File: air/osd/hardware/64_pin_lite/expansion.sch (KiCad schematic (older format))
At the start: 7 parts, among them P11 CONN_1, P13 CONN_1, P2 CONN_20, P3 CONN_20

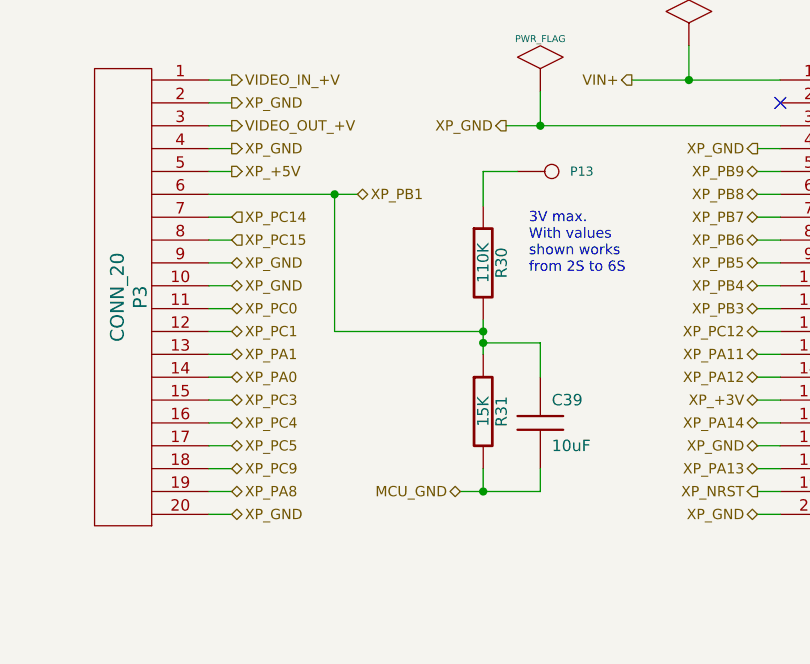
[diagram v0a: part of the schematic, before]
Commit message: hopefully finished
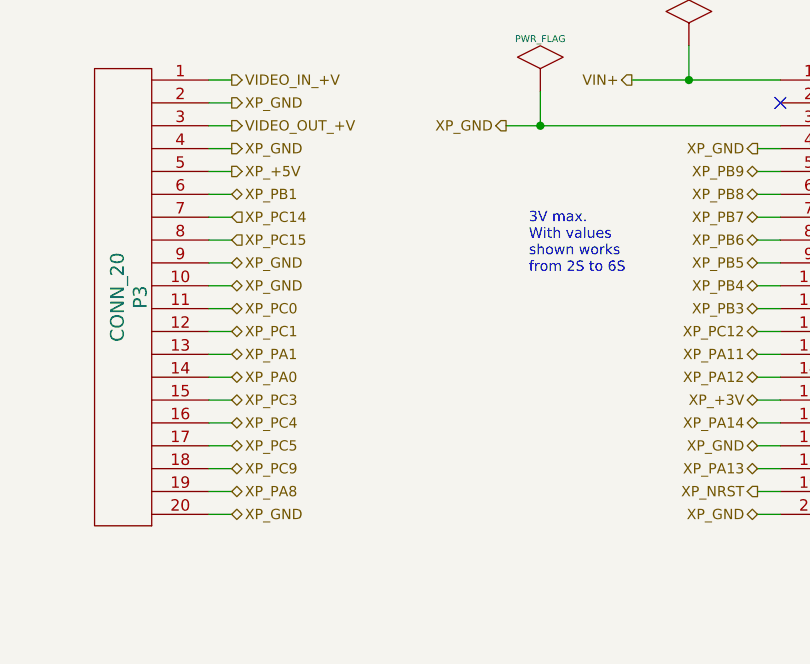
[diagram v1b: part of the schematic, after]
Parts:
- removed C39: 10uF, symbol C
- removed P13: CONN_1, symbol CONN_1
- removed R30: 110K, symbol R
- removed R31: 15K, symbol R
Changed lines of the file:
@@
-EESchema Schematic File Version 2  date Wed 11 Mar 2015 10:11:51 GMT
+EESchema Schematic File Version 2  date Wed 11 Mar 2015 17:51:25 GMT
 LIBS:lm358
 LIBS:conn_6
@@
 Comment4 ""
 $EndDescr
-$Comp
-L CONN_1 P13
-U 1 1 54FDC7F4
-P 5600 2900
-F 0 "P13" H 5680 2900 40  0000 L CNN
-F 1 "CONN_1" H 5600 2955 30  0001 C CNN
-	1    5600 2900
-	1    0    0    -1
-$EndComp
+Text HLabel 4200 3000 2    45   BiDi ~ 0
+XP_PB1
 Wire Wire Line
 	6600 3400 6500 3400
@@
 Wire Wire Line
 	6600 1750 6600 1800
-Connection ~ 5300 4300
-Wire Wire Line
-	5550 4200 5550 4300
-Wire Wire Line
-	5550 4300 5200 4300
-Wire Wire Line
-	5300 4200 5300 4300
-Wire Wire Line
-	5300 3550 5300 3700
 Wire Wire Line
 	6500 4300 6600 4300
@@
 	4100 3200 4200 3200
 Wire Wire Line
-	4750 3000 4100 3000
+	4200 3000 4100 3000
 Connection ~ 6200 2500
 Wire Wire Line
@@
 Wire Wire Line
 	6500 4400 6600 4400
-Wire Wire Line
-	5450 2900 5300 2900
-Wire Wire Line
-	5300 2900 5300 3050
-Wire Wire Line
-	5300 3650 5550 3650
-Wire Wire Line
-	5550 3650 5550 3800
-Connection ~ 5300 3650
-Wire Wire Line
-	5300 3600 4650 3600
-Connection ~ 5300 3600
-Wire Wire Line
-	4650 3600 4650 3000
-Connection ~ 4650 3000
 Wire Wire Line
 	4100 3400 4200 3400
@@
 Text Notes 5500 3350 0    45   ~ 0
 3V max. \nWith values \nshown works \nfrom 2S to 6S\n
-$Comp
-L C C39
-U 1 1 547ED333
-P 5550 4000
-F 0 "C39" H 5600 4100 50  0000 L CNN
-F 1 "10uF" H 5600 3900 50  0000 L CNN
-	1    5550 4000
-	1    0    0    -1
-$EndComp
-Text HLabel 5200 4300 0    45   BiDi ~ 0
-MCU_GND
-$Comp
-L R R31
-U 1 1 547ED2AB
-P 5300 3950
-F 0 "R31" V 5380 3950 50  0000 C CNN
-F 1 "15K" V 5300 3950 50  0000 C CNN
-	1    5300 3950
-	1    0    0    -1
-$EndComp
-$Comp
-L R R30
-U 1 1 547ED2A5
-P 5300 3300
-F 0 "R30" V 5380 3300 50  0000 C CNN
-F 1 "110K" V 5300 3300 50  0000 C CNN
-	1    5300 3300
-	1    0    0    -1
-$EndComp
 Text HLabel 6500 4400 0    45   BiDi ~ 0
 XP_GND
@@
 XP_GND
 $Comp
-L PWR_FLAG #FLG3
+L PWR_FLAG #FLG03
 U 1 1 5474845E
 P 5550 2550
-F 0 "#FLG3" H 5550 2820 30  0001 C CNN
+F 0 "#FLG03" H 5550 2820 30  0001 C CNN
 F 1 "PWR_FLAG" H 5550 2780 30  0000 C CNN
 	1    5550 2550
@@
 $EndComp
 $Comp
-L PWR_FLAG #FLG4
+L PWR_FLAG #FLG04
 U 1 1 54748449
 P 6200 2350
-F 0 "#FLG4" H 6200 2620 30  0001 C CNN
+F 0 "#FLG04" H 6200 2620 30  0001 C CNN
 F 1 "PWR_FLAG" H 6200 2580 30  0000 C CNN
 	1    6200 2350
@@
 Text HLabel 4200 4400 2    45   BiDi ~ 0
 XP_GND
-Text HLabel 4750 3000 2    45   BiDi ~ 0
-XP_PB1
 $EndSCHEMATC
